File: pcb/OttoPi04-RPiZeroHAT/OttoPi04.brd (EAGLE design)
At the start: 63.5 x 48.3 mm, 25 parts

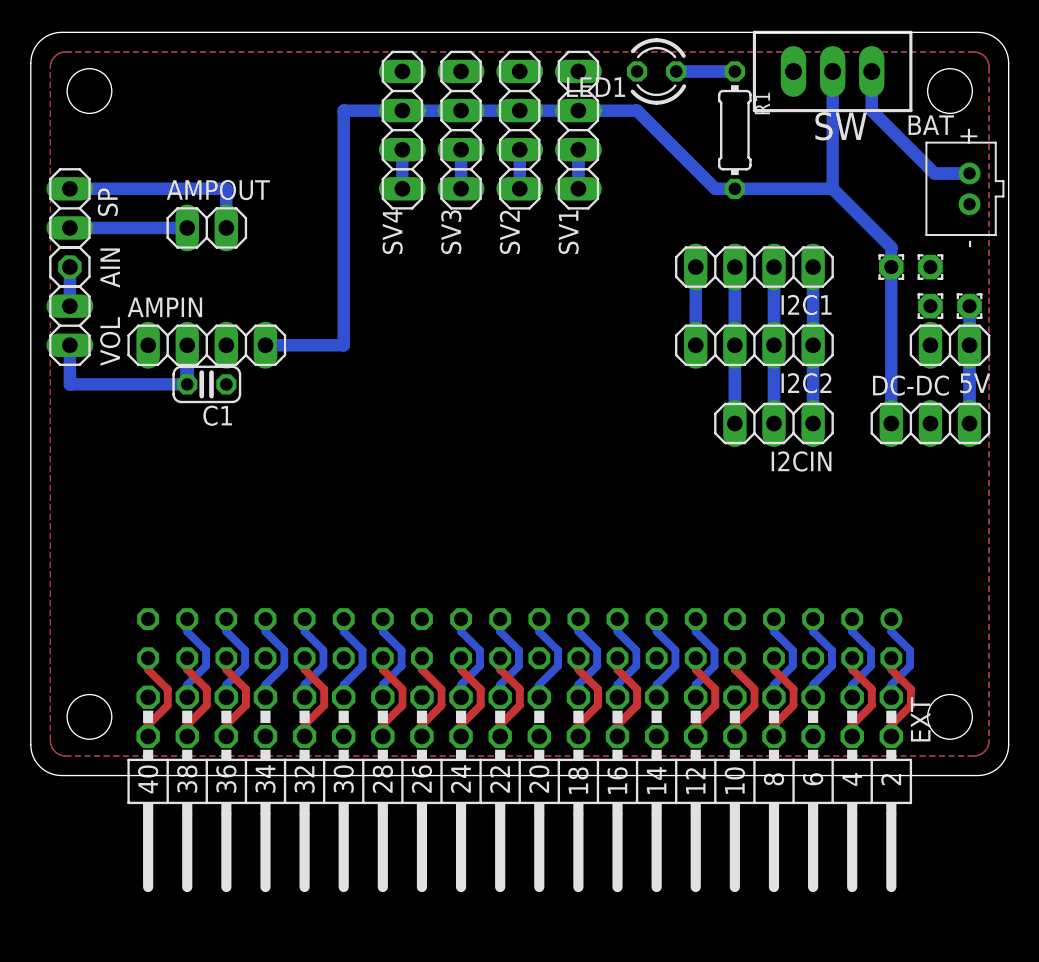
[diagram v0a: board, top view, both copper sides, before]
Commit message: pcb/OttoPi04-RPiZeroHAT
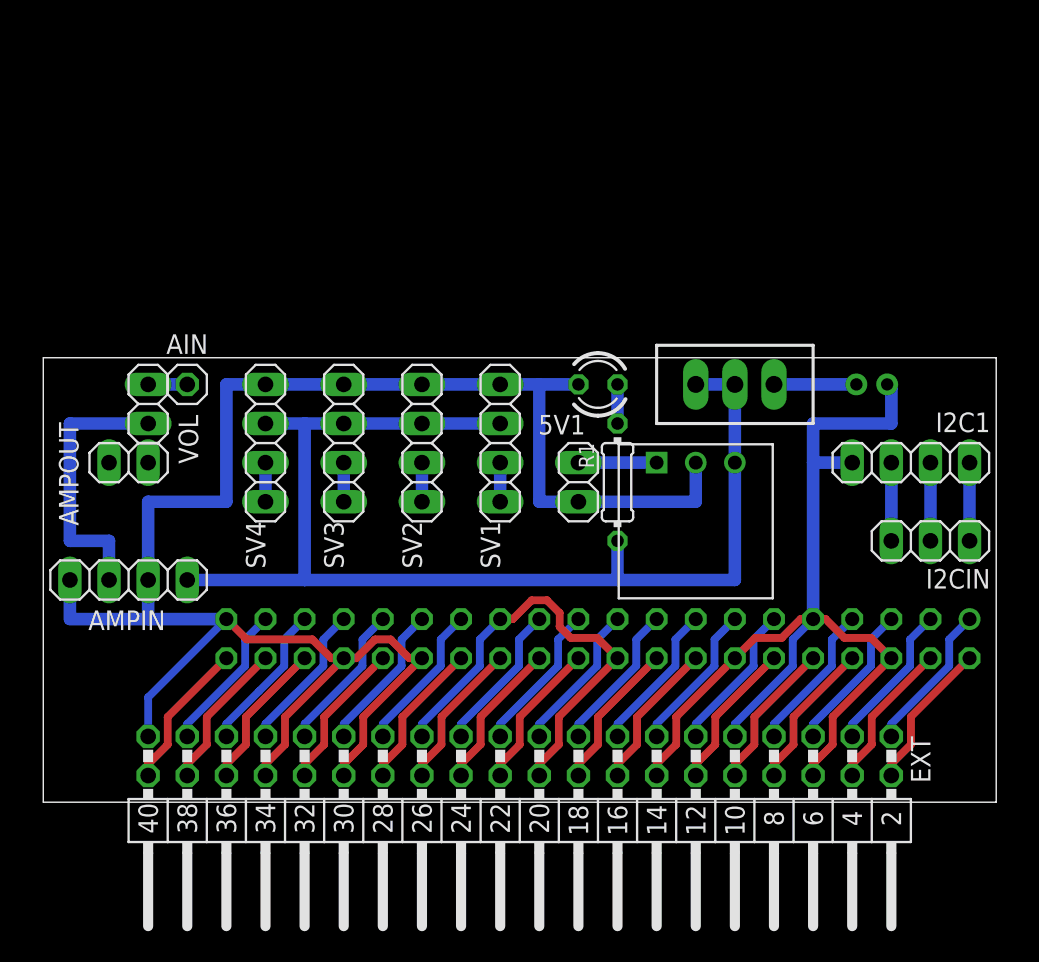
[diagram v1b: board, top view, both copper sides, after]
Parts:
- removed 5V, SP: (no value), pinhead:1X02
- removed 5V_A: 5V, wirepad:1,6/0,9
- removed BAT_B, G: (no value), wirepad:1,6/0,9
- removed C1: (no value), rcl:C025-024X044
- removed DC-DC: (no value), pinhead:1X03
- removed GND_A: G, wirepad:1,6/0,9
- removed I2C2: (no value), pinhead:1X04
- added 5V1: (no value), pinhead:1X02
- added DC/DC1: DC/DC-03_5V_480MA, ytani1:DC/DC:480MA
- R1: value (none) -> 1K
- moved R1 24.1 mm to (38.1, 21.6)
- moved SV4 22.2 mm to (15.2, 24.1)
- moved SV3 21.7 mm to (20.3, 24.1)
- moved SV2 21.3 mm to (25.4, 24.1)
- moved SW 21.3 mm to (45.7, 27.9)
- moved SV1 20.9 mm to (30.5, 24.1)
- moved LED1 20.7 mm to (36.8, 27.9)
- moved I2C1 16.3 mm to (57.1, 22.9)
- moved AMPIN 16.1 mm to (6.35, 15.2)
- moved AMPOUT 16.1 mm to (6.35, 22.9), turned to 180 degrees
- moved BAT 14.2 mm to (54.6, 27.9), flipped to the bottom, turned to 0 degrees
- moved I2CIN 12.7 mm to (58.4, 17.8)
- moved AIN 10.8 mm to (10.2, 27.9), turned to 90 degrees
- moved VOL 7.18 mm to (7.62, 26.7)
- moved RPI 5.08 mm to (36.8, 11.4)
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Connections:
- removed net BAT+: AMPIN.4, BAT_B.1, DC-DC.1, R1.2, SV1.2, SV2.2, SV3.2, SV4.2, SW.2
- removed net SP+: AMPOUT.1, SP.1
- removed net SP-: AMPOUT.2, SP.2
- new net V+: AMPIN.4, DC/DC1.3, R1.2, SV1.2, SV2.2, SV3.2, SV4.2, SW.2, SW.3
- net +3V3: no longer I2C2.1
- net +5V: now also 5V1.2, DC/DC1.1; no longer 5V.1, 5V_A.1, DC-DC.3
- net AIN2: no longer C1.2
- net GND: now also 5V1.1, DC/DC1.2; no longer 5V.2, C1.1, DC-DC.2, G.1, GND_A.1, I2C2.4
- net SCL: no longer I2C2.3
- net SDL: no longer I2C2.2
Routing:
- net GND: track 5.38 -> 214.2 mm
- net V+: track 0.00 -> 78.7 mm
- net BAT+: track 78.6 -> 0.00 mm
- net SP-: track 12.7 -> 0.00 mm
- net SP+: track 7.62 -> 0.00 mm
- net +4V_S: track 10.6 -> 5.35 mm
- net SDL: track 10.2 -> 5.08 mm
- net SCL: track 10.2 -> 5.08 mm
- net +3V3: track 10.2 -> 5.08 mm
- net AIN2: track 12.7 -> 17.8 mm
- net SDA-S: track 6.09 -> 9.72 mm
- net GPIO10: track 6.09 -> 9.72 mm
- net GPIO11: track 6.09 -> 9.72 mm
- net GPIO6: track 6.09 -> 9.72 mm
- net SCL-S: track 6.09 -> 9.72 mm
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- removed copper zone on layer 1, net GND
- removed copper zone on layer 16, net GND
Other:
- board size 63.5 x 48.3 mm -> 61.9 x 28.9 mm

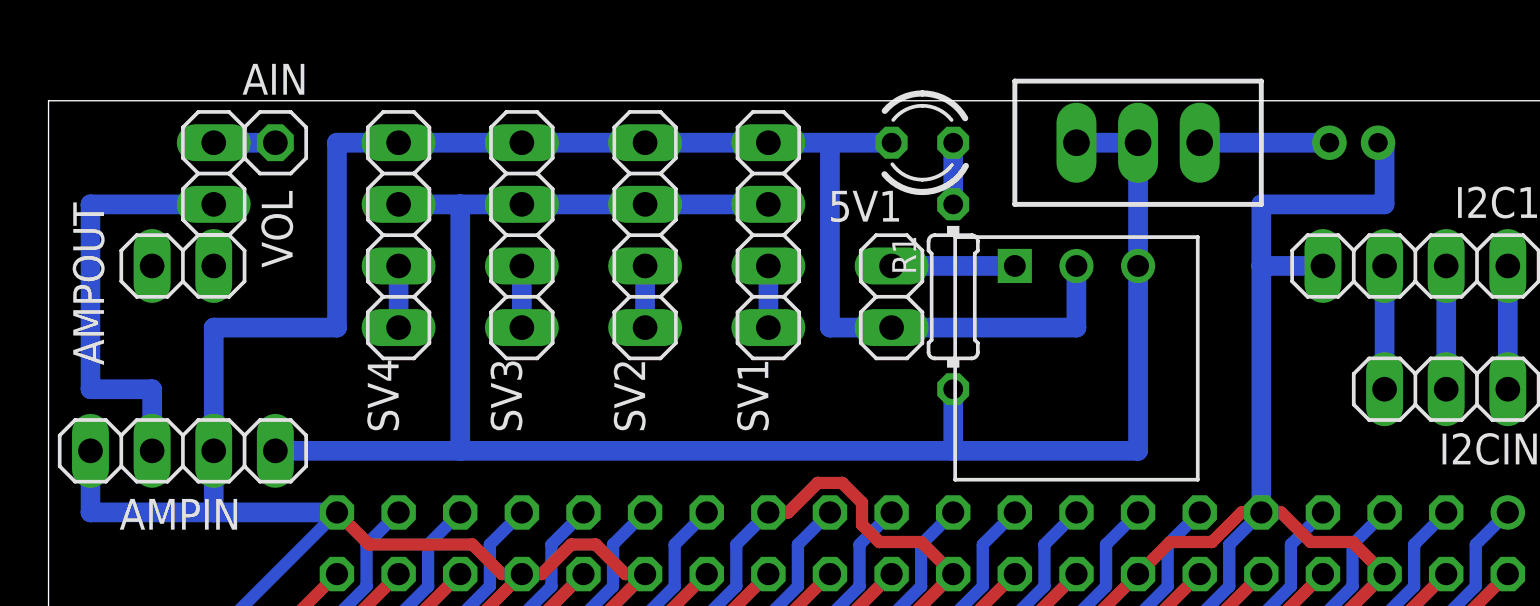
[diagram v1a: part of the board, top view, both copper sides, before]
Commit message: update
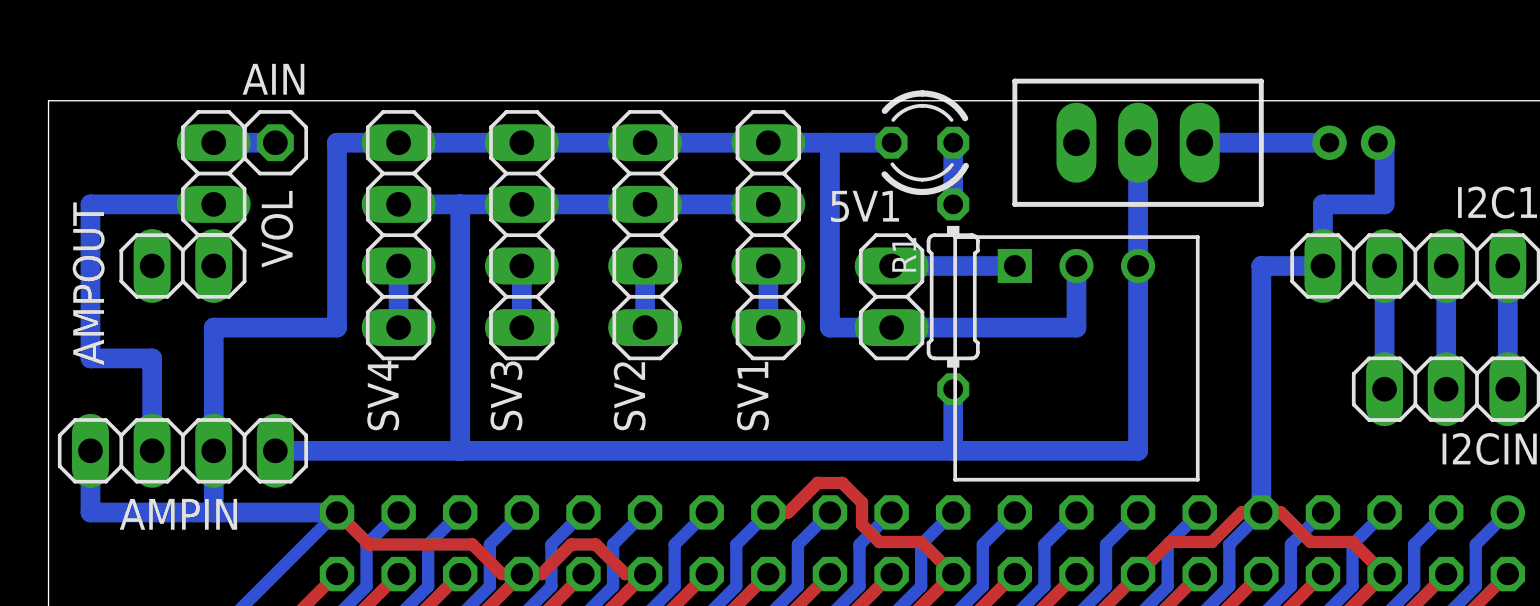
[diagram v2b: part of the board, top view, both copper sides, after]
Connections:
- net V+: no longer SW.3
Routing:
- net GND: track 214.2 -> 211.7 mm
- net V+: track 78.7 -> 76.2 mm
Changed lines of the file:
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@@
 <?xml version="1.0" encoding="utf-8"?>
 <!DOCTYPE eagle SYSTEM "eagle.dtd">
-<eagle version="9.6.0">
+<eagle version="9.6.2">
 <drawing>
 <settings>
@@
 <wire x1="33.02" y1="27.94" x2="35.56" y2="27.94" width="0.8128" layer="16"/>
 <wire x1="50.8" y1="12.7" x2="50.8" y2="22.86" width="0.8128" layer="16"/>
-<wire x1="50.8" y1="22.86" x2="50.8" y2="25.4" width="0.8128" layer="16"/>
-<wire x1="50.8" y1="25.4" x2="55.88" y2="25.4" width="0.8128" layer="16"/>
+<wire x1="53.34" y1="22.86" x2="53.34" y2="25.4" width="0.8128" layer="16"/>
+<wire x1="53.34" y1="25.4" x2="55.88" y2="25.4" width="0.8128" layer="16"/>
 <wire x1="55.88" y1="25.4" x2="55.88" y2="27.67" width="0.8128" layer="16"/>
 <wire x1="50.8" y1="22.86" x2="53.34" y2="22.86" width="0.8128" layer="16"/>
@@
 <contactref element="VOL" pad="2"/>
 <wire x1="7.62" y1="25.4" x2="2.54" y2="25.4" width="0.8128" layer="16"/>
-<wire x1="2.54" y1="25.4" x2="2.54" y2="17.78" width="0.8128" layer="16"/>
-<wire x1="2.54" y1="17.78" x2="5.08" y2="17.78" width="0.8128" layer="16"/>
-<wire x1="5.08" y1="17.78" x2="5.08" y2="15.24" width="0.8128" layer="16"/>
+<wire x1="2.54" y1="25.4" x2="2.54" y2="19.05" width="0.8128" layer="16"/>
+<wire x1="2.54" y1="19.05" x2="5.08" y2="19.05" width="0.8128" layer="16"/>
+<wire x1="5.08" y1="19.05" x2="5.08" y2="15.24" width="0.8128" layer="16"/>
 </signal>
 <signal name="AIN1">
@@
 <contactref element="SW" pad="2"/>
 <contactref element="R1" pad="2"/>
-<contactref element="SW" pad="3"/>
-<wire x1="45.72" y1="27.94" x2="43.18" y2="27.94" width="0.8128" layer="16"/>
 <contactref element="SV1" pad="2"/>
 <contactref element="SV2" pad="2"/>
